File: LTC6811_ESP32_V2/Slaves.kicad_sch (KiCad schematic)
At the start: 3 parts, among them J7 B2P-VH-B, J9 B2P-VH-B

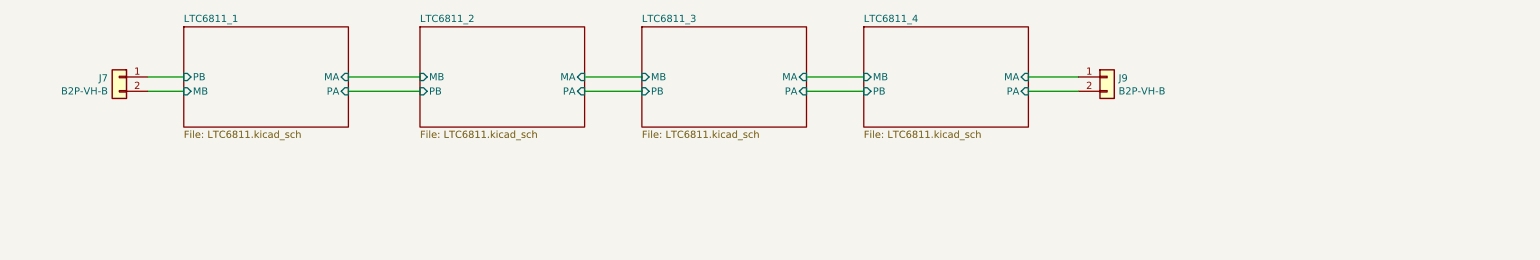
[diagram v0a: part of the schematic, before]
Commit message: Add files via upload
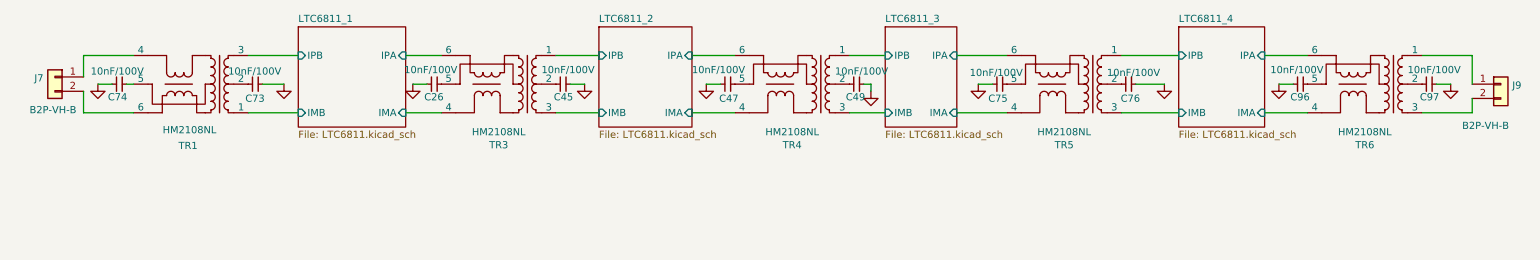
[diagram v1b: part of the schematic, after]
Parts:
- added C26, C45, C47, C49, C73, C74, C75, C76, C96, C97: 10nF/100V, Capacitor_SMD:C_0402_1005Metric, symbol Library:C
- added TR1, TR3, TR4, TR5, TR6: HM2108NL, Transformer_SMD:HM2108NL, symbol Library:HM2108NL
- J7, J9: symbol Connector_Generic:Conn_01x02 -> Library:Conn_01x02
- LOGO2: symbol Graphic:Logo_Tetra -> Library:Logo_Tetra
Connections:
- net LTC6811_1/MB: no longer names the net of J7.2 (Pin_2)
- net LTC6811_1/MB: now also TR1.6
- net LTC6811_1/PB: no longer names the net of J7.1 (Pin_1)
- net LTC6811_1/PB: now also TR1.4
- net LTC6811_4/MA: no longer names the net of J9.1 (Pin_1)
- net LTC6811_4/MA: now also TR6.1
- net LTC6811_4/PA: no longer names the net of J9.2 (Pin_2)
- net LTC6811_4/PA: now also TR6.3
- new net: C73.2, TR1.2
- new net: C74.1, TR1.5
- new net: C76.1, TR5.2
- new net: C75.1, TR5.5
- new net: C96.1, TR6.5
- new net: C97.1, TR6.2
- new net: C26.1, TR3.5
- new net: C45.1, TR3.2
- new net: C49.1, TR4.2
- new net: C47.1, TR4.5
- new net GND_PACK: C26.2, C45.2, C47.2, C49.2, C73.1, C74.2, C75.2, C76.2, C96.2, C97.2
- new net LTC6811_1/IMA: TR3.4
- new net LTC6811_1/IMB: TR1.1
- new net LTC6811_1/IPA: TR3.6
- new net LTC6811_1/IPB: TR1.3
- new net LTC6811_2/IMA: TR4.4
- new net LTC6811_2/IMB: TR3.3
- new net LTC6811_2/IPA: TR4.6
- new net LTC6811_2/IPB: TR3.1
- new net LTC6811_3/IMA: TR5.4
- new net LTC6811_3/IMB: TR4.3
- new net LTC6811_3/IPA: TR5.6
- new net LTC6811_3/IPB: TR4.1
- new net LTC6811_4/IMA: TR6.4
- new net LTC6811_4/IMB: TR5.3
- new net LTC6811_4/IPA: TR6.6
- new net LTC6811_4/IPB: TR5.1
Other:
- sheet LTC6811_1 ports: added IMA, IMB, IPA, IPB; removed MA, MB, PA, PB
- sheet LTC6811_2 ports: added IMA, IMB, IPA, IPB; removed MA, MB, PA, PB
- sheet LTC6811_3 ports: added IMA, IMB, IPA, IPB; removed MA, MB, PA, PB
- sheet LTC6811_4 ports: added IMA, IMB, IPA, IPB; removed MA, MB, PA, PB
- moved on the sheet: J7, J9
